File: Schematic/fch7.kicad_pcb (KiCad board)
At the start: 4 copper layers, 42 x 42 mm, 151 parts, among them IC1 MP9943AGQ-Z, IC2 MP9943AGQ-Z, IC3 STM32H743VIT6, IC4 ICM-42688-P, IC5 MPU-6500, J10 PIN2216, J11 PIN2216, J12 PIN2216, J2 PIN2216, J3 PIN2216, J4 PIN2216, J5 PIN2216, J6 PIN2216, J7 PIN2216, J8 PIN2216, J9 PIN2216, SW1 TS24CA, SW2 TS24CA, U1 ME6217C33M5G, U10 HDGC1002WR-S-4P, U11 HDGC1002WR-S-4P, U12 E28-2G4M27SX, U13 ESP-01F-2M, U14 HDGC1002WR-S-4P, U15 HDGC1002WR-S-6P, U16 HDGC1002WR-S-8P, U17 HDGC1002WR-S-8P, U2 ME6217C33M5G, U3 LDO-1.8v, U4 QMC5883L, U5 SPL06-001, U6 CSNP1GCR01-BOW, U7 HDGC1002WR-S-4P, U8 HDGC1002WR-S-4P, U9 HDGC1002WR-S-4P, Y1 8MHz

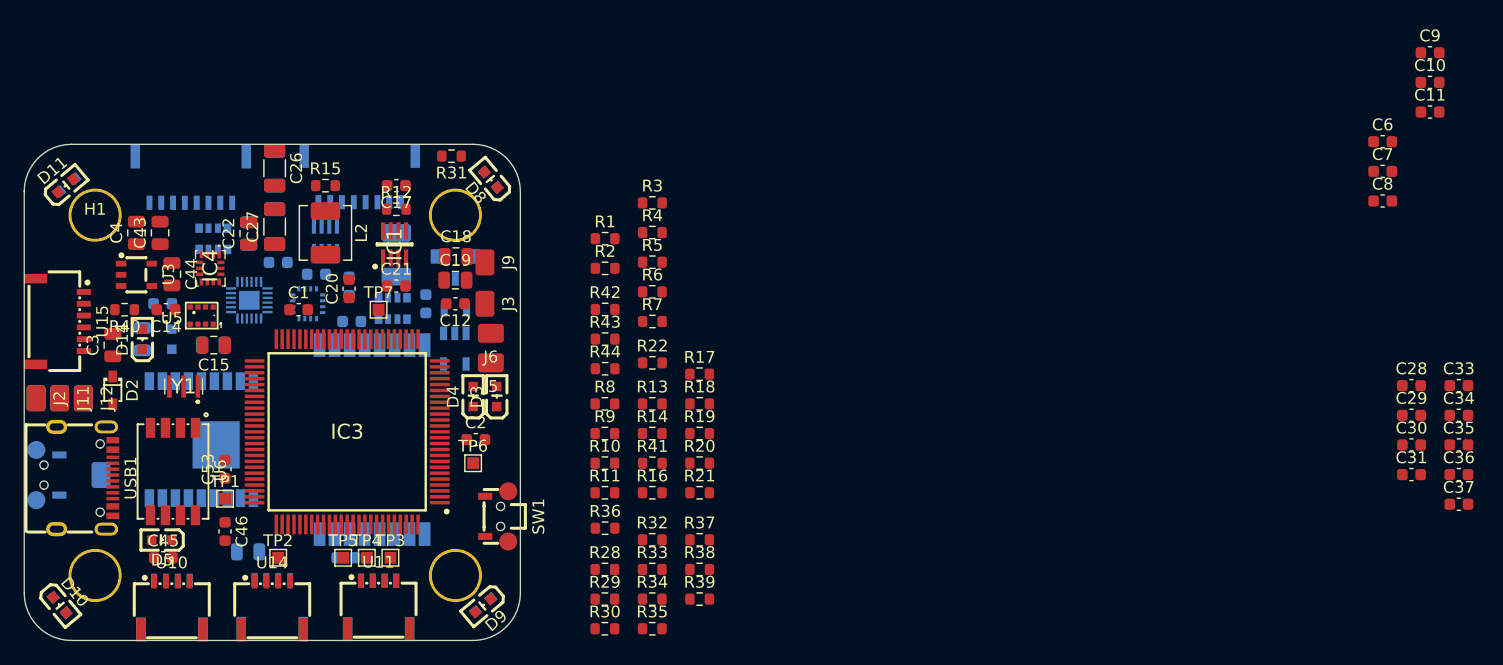
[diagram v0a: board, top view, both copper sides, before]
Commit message: finised capacitor placement
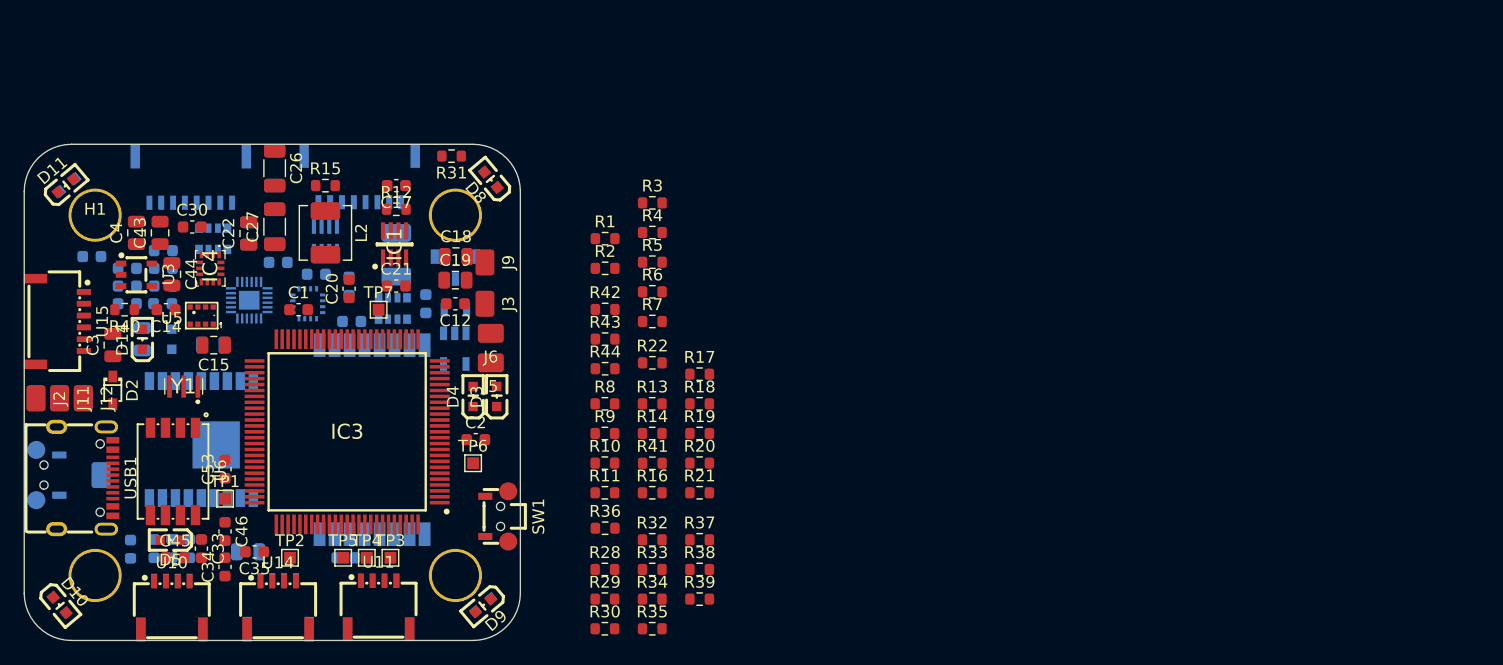
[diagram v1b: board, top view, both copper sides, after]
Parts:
- C10, C11, C28, C29, C31, C36, C37, C6, C7, C8, C9: moved to B.Cu
- moved C31 113.2 mm to (68.7, 69.5)
- moved C37 112.5 mm to (72.0, 94.3), turned to 90 degrees
- moved C36 110.6 mm to (74.0, 94.2), turned to 90 degrees
- moved C9 109.0 mm to (74.8, 72.0)
- moved C10 108.4 mm to (74.8, 70.5)
- moved C11 107.9 mm to (74.8, 69.0)
- moved C33 107.3 mm to (78.0, 94.2), turned to -90 degrees
- moved C6 106.8 mm to (71.7, 70.5), turned to 180 degrees
- moved C7 106.7 mm to (71.7, 72.0), turned to 180 degrees
- moved C8 106.6 mm to (71.7, 73.5), turned to 180 degrees
- moved C28 105.8 mm to (75.5, 94.2), turned to -90 degrees
- moved C34 105.2 mm to (80.0, 95.8), turned to 90 degrees
- moved C30 104.8 mm to (77.2, 67.0)
- moved C29 104.0 mm to (77.0, 94.2), turned to -90 degrees
- moved C35 102.3 mm to (82.5, 94.5), turned to 180 degrees
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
